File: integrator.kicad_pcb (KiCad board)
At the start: 4 copper layers, 65.5 x 117 mm, 102 parts, among them J1 SJ-3524-SMT, J2 SJ-3524-SMT, J3 SP-3533-02, J4 SP-3533-02, J5 USB4105-GF-A, J6 Conn_ARM_JTAG_SWD_10, J7 test point, SW1 EVQP40B3M, SW2 EVQP40B3M, SW3 EVQP40B3M, SW4 436333033816, U1 XC6415, U2 MCP1700-2302E/TT, U3 LSM6DSO32XTR, U4 NL27WZ16DTT1G, U5 RP2040, U6 IS25WP128F-JBLE, U7 NL27WZ16DTT1G, Y1 Crystal

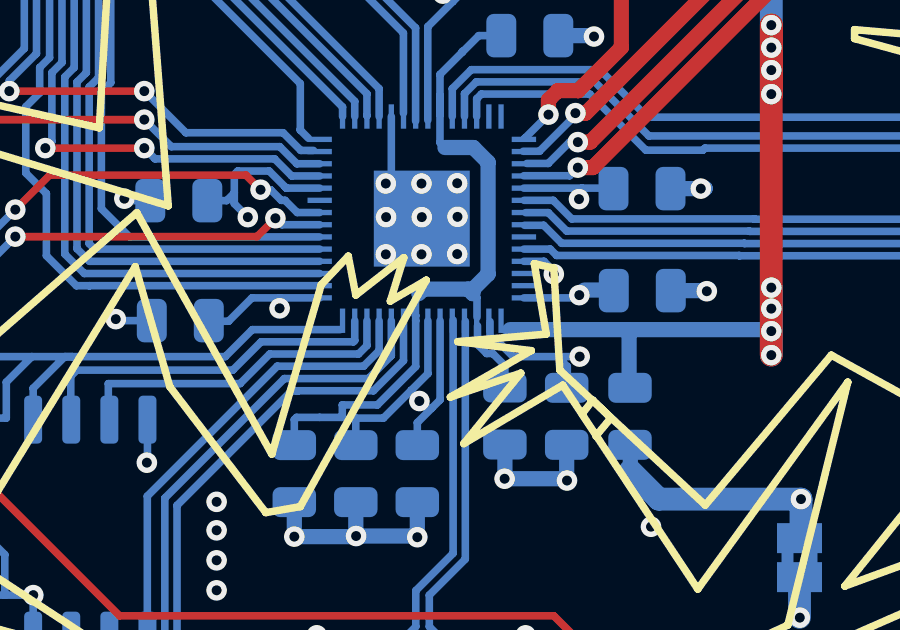
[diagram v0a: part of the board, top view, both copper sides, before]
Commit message: v9 checkpoint/wip
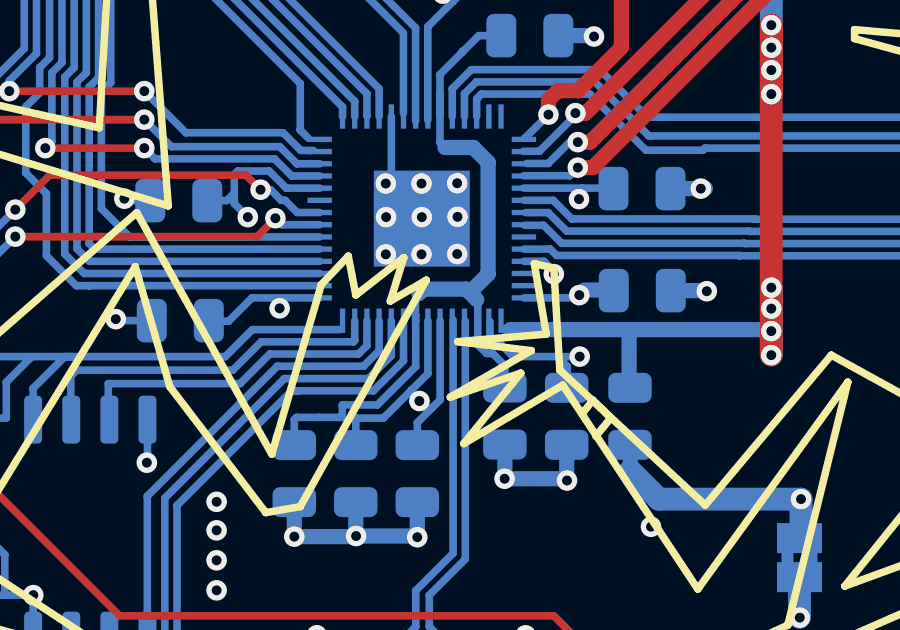
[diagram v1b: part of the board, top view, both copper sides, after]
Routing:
- net VInt: track 25.7 -> 26.2 mm
